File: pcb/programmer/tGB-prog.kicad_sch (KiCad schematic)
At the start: 40 parts, among them J1 ZX62R-B-5P, J2 PROG_PORT, U1 FT2232D, U2 93LC56BT-I/OT, U3 TPS79901DDCR, Y1 NX8045GB-6MHZ-STD-CSF-3

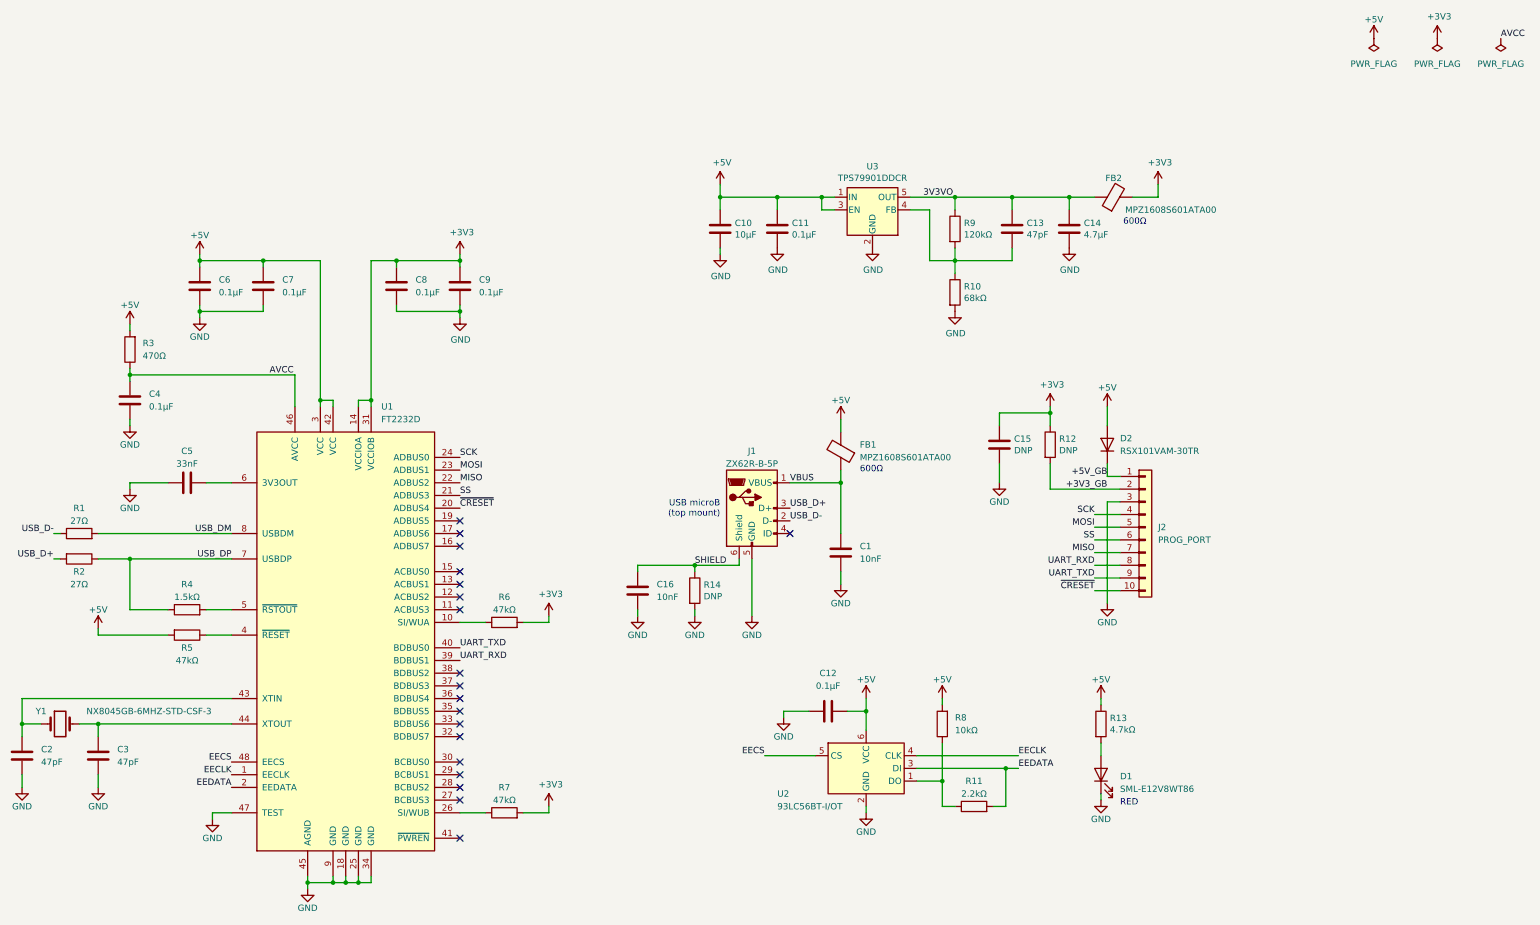
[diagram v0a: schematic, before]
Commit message: add comments
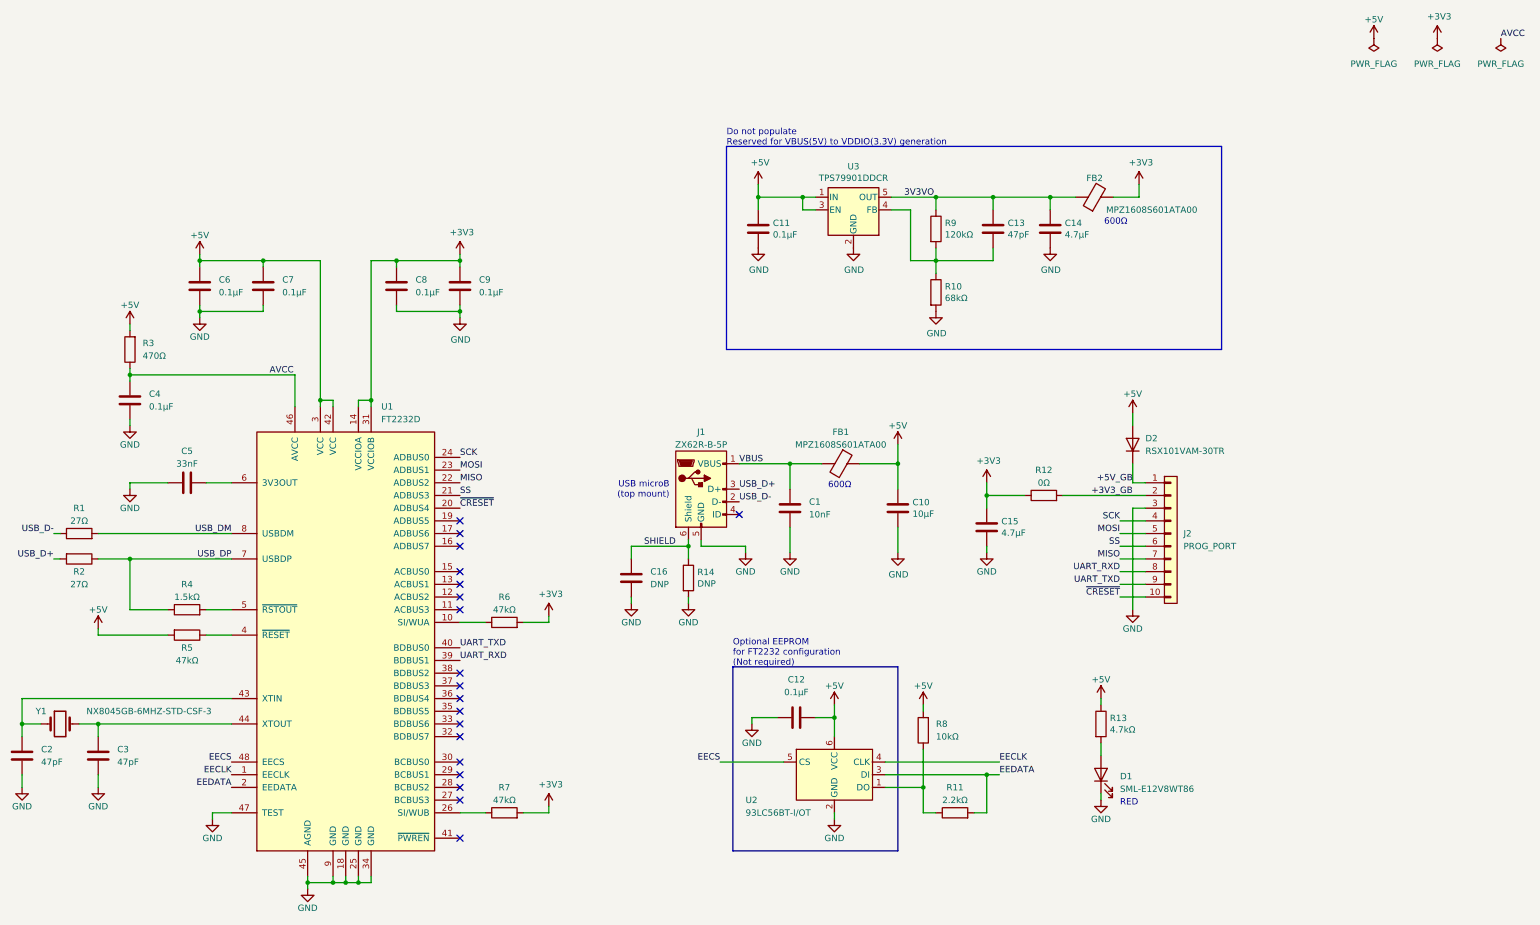
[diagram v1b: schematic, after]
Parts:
- C15: value DNP -> 4.7μF
- C16: value 10nF -> DNP
- R12: value DNP -> 0Ω
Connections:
- net +5V: now also FB1.1; no longer FB1.2
- net VBUS: now also FB1.2; no longer FB1.1
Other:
- note added: "Do not populate Reserved for VBUS(5V) to VDDIO(3.3V) generation"
- note added: "Optional EEPROM for FT2232 configuration (Not required)"
- moved on the sheet: C1, C10, C11, C12, C13, C14, C15, C16, D2, FB1, FB2, J1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
